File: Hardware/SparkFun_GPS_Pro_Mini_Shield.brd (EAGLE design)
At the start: 20.3 x 40.6 mm, 23 parts, among them J1 MICROSD_TINY, U1 GP735, U2 TXB0108, U3 AP2112K-3.3V

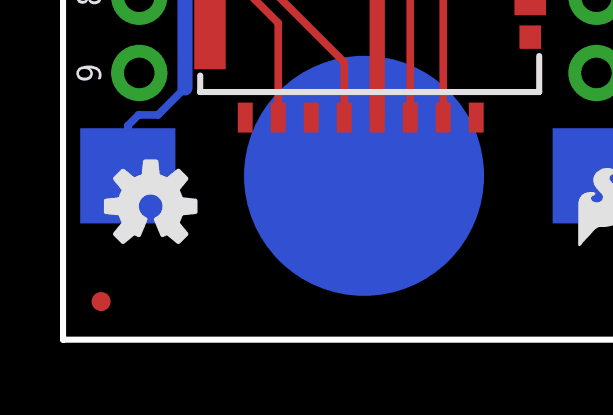
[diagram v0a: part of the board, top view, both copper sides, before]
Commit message: Added board designer name and version number
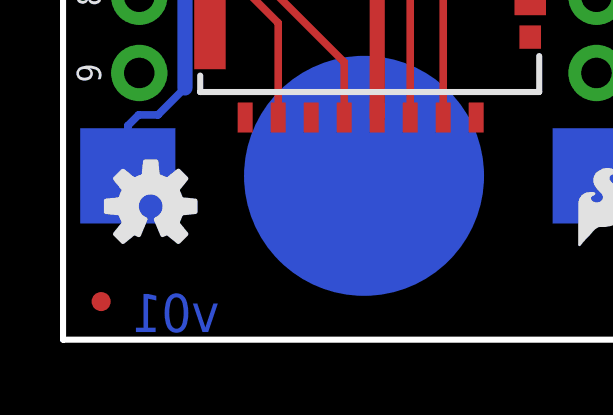
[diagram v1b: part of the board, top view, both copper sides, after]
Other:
- board text added: "v01"
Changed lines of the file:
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@@
 <layer number="45" name="Holes" color="7" fill="1" visible="yes" active="yes"/>
 <layer number="46" name="Milling" color="3" fill="1" visible="no" active="yes"/>
-<layer number="47" name="Measures" color="7" fill="1" visible="yes" active="yes"/>
+<layer number="47" name="Measures" color="7" fill="1" visible="no" active="yes"/>
 <layer number="48" name="Document" color="7" fill="1" visible="no" active="yes"/>
 <layer number="49" name="Reference" color="7" fill="1" visible="no" active="yes"/>
@@
 <text x="13.97" y="38.1" size="0.8128" layer="22" font="vector" ratio="15" rot="MR180" align="bottom-center">3.3V</text>
 <text x="16.129" y="38.1" size="0.8128" layer="22" font="vector" ratio="15" rot="MR270" align="center-left">GND</text>
+<text x="5.207" y="0.254" size="1.27" layer="16" font="vector" ratio="15" rot="MR0">v01</text>
 </plain>
 <attributes>
